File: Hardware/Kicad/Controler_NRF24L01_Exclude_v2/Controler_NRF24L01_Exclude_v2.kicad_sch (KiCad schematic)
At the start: 38 parts, among them J1 Conn_01x02, J2 Conn_02x07_Odd_Even, J3 Conn_01x03, J4 Conn_01x03, SW1 SW_Push, SW10 SW_Push, SW11 SW_DIP_x01, SW13 SW_DIP_x01, SW2 SW_Push, SW3 SW_Push, SW4 SW_Push, SW5 SW_Push, SW6 SW_Push, SW7 SW_Push, SW7 SW_SPST, SW8 SW_Push, SW9 SW_Push, U1 STM32L412KBTx, U2 MIC5219-3.3YMM, U2 nRF24_Full

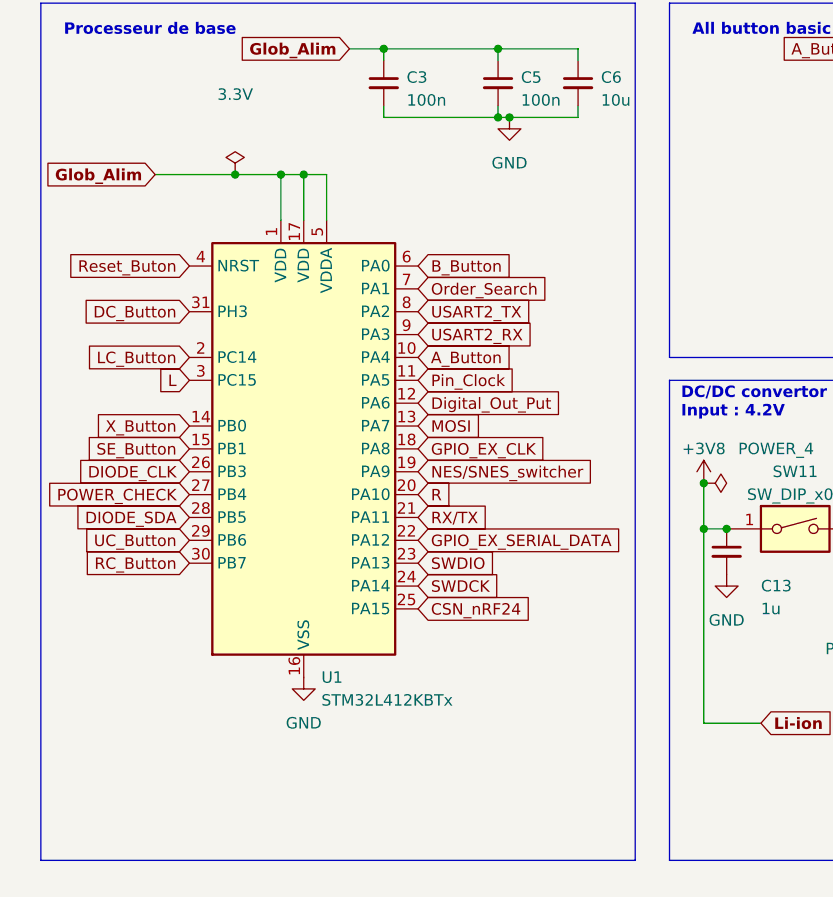
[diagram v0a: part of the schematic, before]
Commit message: V.2 controler
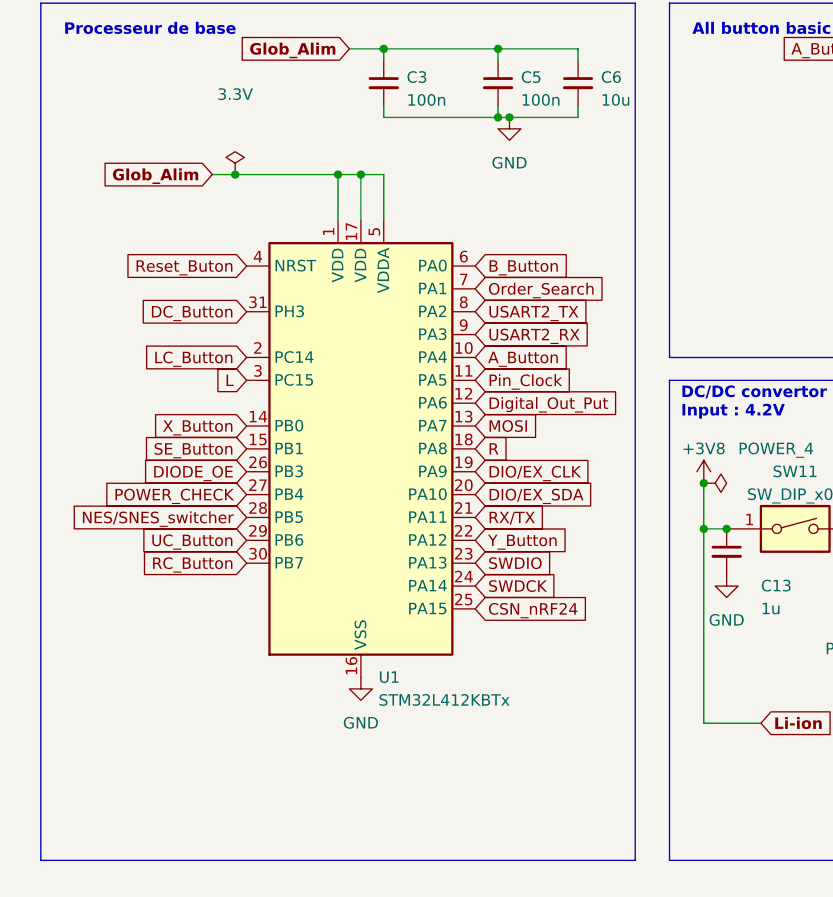
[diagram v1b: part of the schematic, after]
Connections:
- net DIODE_SDA is gone; now on net NES/SNES_switcher: U1.28 (PB5)
- net GPIO_EX_CLK is gone; now on net R: U1.18 (PA8)
- net GPIO_EX_SERIAL_DATA is gone; now on net Y_Button: U1.22 (PA12)
- net NES/SNES_switcher: no longer U1.19 (PA9)
- net R: no longer U1.20 (PA10)
- net DIODE_CLK renamed DIODE_OE
- new net DIO/EX_CLK: U1.19 (PA9)
- new net DIO/EX_SDA: U1.20 (PA10)
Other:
- moved on the sheet: U1

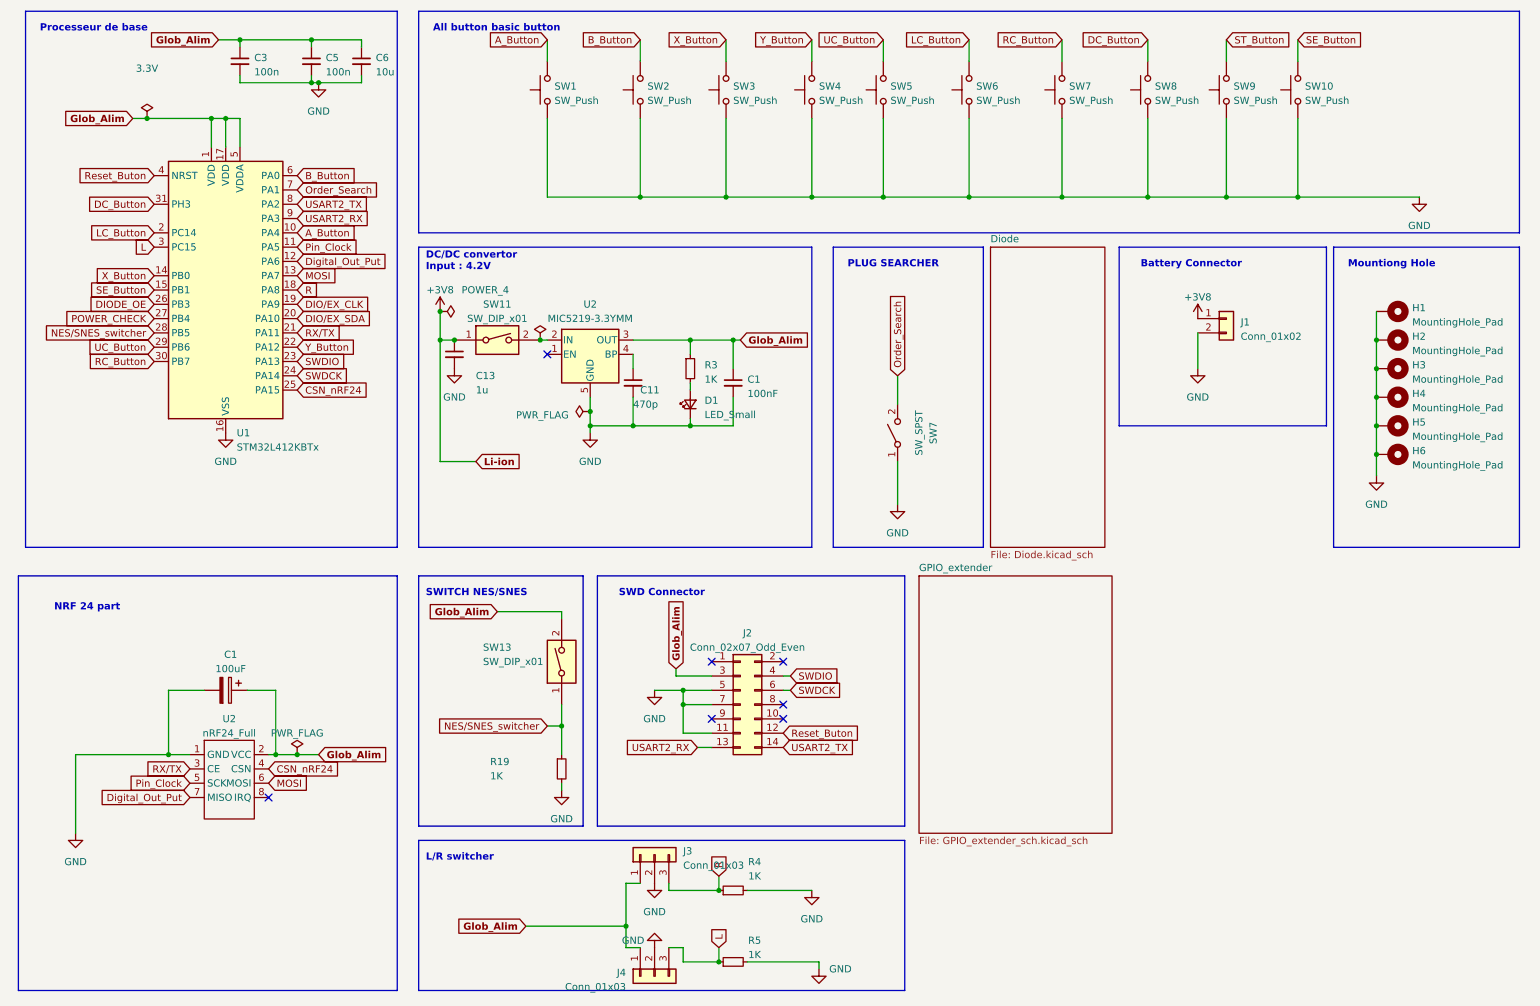
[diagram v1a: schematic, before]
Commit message: V.2 controler
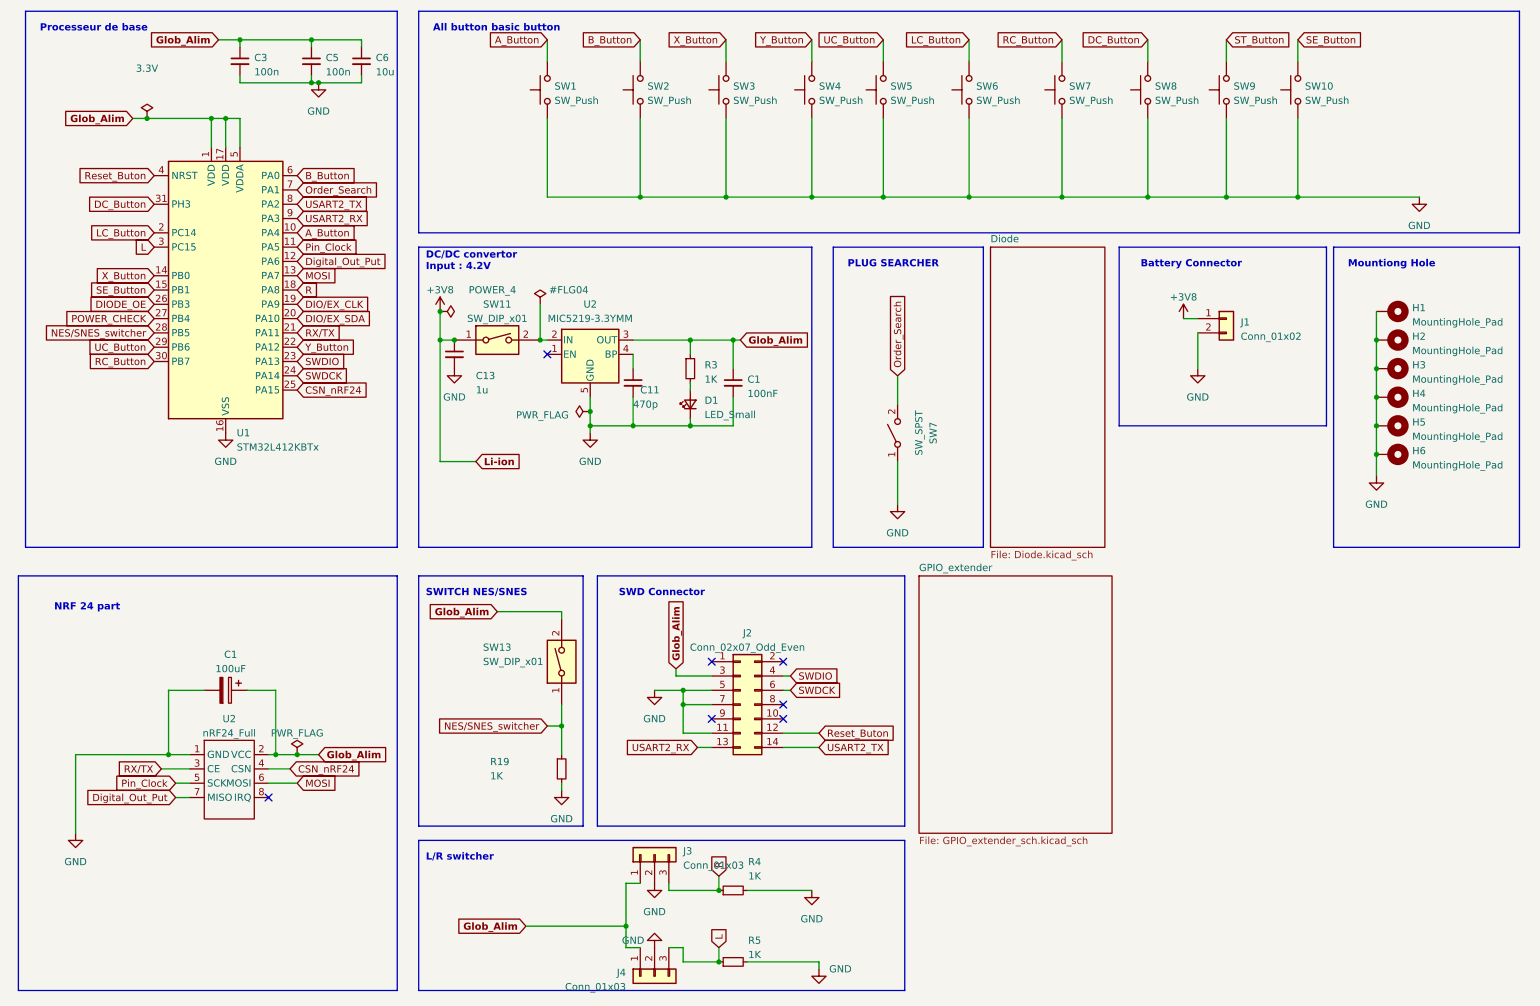
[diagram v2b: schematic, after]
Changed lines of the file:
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@@
+    (stroke (width 0) (type default))
+  )
+  (wire (pts (xy 39.37 149.86) (xy 44.45 149.86))
     (stroke (width 0) (type default))
   )
@@
     (stroke (width 0) (type default))
   )
+  (wire (pts (xy 63.5 152.4) (xy 58.42 152.4))
+    (stroke (width 0) (type default))
+  )
   (wire (pts (xy 143.51 171.45) (xy 154.94 171.45))
     (stroke (width 0) (type default))
@@
     (stroke (width 0) (type default))
   )
+  (wire (pts (xy 62.23 149.86) (xy 58.42 149.86))
+    (stroke (width 0) (type default))
+  )
   (wire (pts (xy 133.35 88.9) (xy 140.97 88.9))
     (stroke (width 0) (type default))
@@
     (stroke (width 0) (type default))
   )
+  (wire (pts (xy 41.91 154.94) (xy 44.45 154.94))
+    (stroke (width 0) (type default))
+  )
   (polyline (pts (xy 158.75 57.15) (xy 158.75 110.49))
     (stroke (width 0) (type default))
@@
     (stroke (width 0) (type default))
   )
+  (wire (pts (xy 41.91 152.4) (xy 44.45 152.4))
+    (stroke (width 0) (type default))
+  )
+  (wire (pts (xy 220.98 69.85) (xy 223.52 69.85))
+    (stroke (width 0) (type default))
+  )
   (wire (pts (xy 140.97 73.66) (xy 142.24 73.66))
     (stroke (width 0) (type default))
@@
     (stroke (width 0) (type default))
   )
+  (wire (pts (xy 156.21 146.05) (xy 149.86 146.05))
+    (stroke (width 0) (type default))
+  )
   (wire (pts (xy 228.6 20.32) (xy 228.6 24.13))
     (stroke (width 0) (type default))
@@
     (stroke (width 0) (type default))
   )
+  (wire (pts (xy 156.21 143.51) (xy 149.86 143.51))
+    (stroke (width 0) (type default))
+  )
   (wire (pts (xy 223.52 72.39) (xy 223.52 78.74))
     (stroke (width 0) (type default))
@@
   )
   (wire (pts (xy 104.14 177.8) (xy 121.92 177.8))
+    (stroke (width 0) (type default))
+  )
+  (wire (pts (xy 106.68 67.31) (xy 106.68 73.66))
     (stroke (width 0) (type default))
   )
@@
     )
   )
-  (global_label "Reset_Buton " (shape input) (at 149.86 143.51 0) (fields_autoplaced)
-    (effects (font (size 1.27 1.27)) (justify left))
-    (property "Intersheetrefs" "${INTERSHEET_REFS}" (at 165.1391 143.51 0)
+  (global_label "Reset_Buton " (shape input) (at 156.21 143.51 0) (fields_autoplaced)
+    (effects (font (size 1.27 1.27)) (justify left))
+    (property "Intersheetrefs" "${INTERSHEET_REFS}" (at 171.4891 143.51 0)
       (effects (font (size 1.27 1.27)) (justify left) hide)
     )
@@
     )
   )
-  (global_label "RX{slash}TX" (shape input) (at 44.45 149.86 180) (fields_autoplaced)
-    (effects (font (size 1.27 1.27)) (justify right))
-    (property "Intersheetrefs" "${INTERSHEET_REFS}" (at 35.5571 149.86 0)
+  (global_label "RX{slash}TX" (shape input) (at 39.37 149.86 180) (fields_autoplaced)
+    (effects (font (size 1.27 1.27)) (justify right))
+    (property "Intersheetrefs" "${INTERSHEET_REFS}" (at 30.4771 149.86 0)
       (effects (font (size 1.27 1.27)) (justify right) hide)
     )
@@
     )
   )
-  (global_label "USART2_TX" (shape input) (at 149.86 146.05 0) (fields_autoplaced)
-    (effects (font (size 1.27 1.27)) (justify left))
-    (property "Intersheetrefs" "${INTERSHEET_REFS}" (at 162.9862 146.05 0)
-      (effects (font (size 1.27 1.27)) (justify left) hide)
-    )
-  )
-  (global_label "Pin_Clock" (shape input) (at 44.45 152.4 180) (fields_autoplaced)
-    (effects (font (size 1.27 1.27)) (justify right))
-    (property "Intersheetrefs" "${INTERSHEET_REFS}" (at 32.3519 152.4 0)
+  (global_label "USART2_TX" (shape input) (at 156.21 146.05 0) (fields_autoplaced)
+    (effects (font (size 1.27 1.27)) (justify left))
+    (property "Intersheetrefs" "${INTERSHEET_REFS}" (at 169.3362 146.05 0)
+      (effects (font (size 1.27 1.27)) (justify left) hide)
+    )
+  )
+  (global_label "Pin_Clock" (shape input) (at 41.91 152.4 180) (fields_autoplaced)
+    (effects (font (size 1.27 1.27)) (justify right))
+    (property "Intersheetrefs" "${INTERSHEET_REFS}" (at 29.8119 152.4 0)
       (effects (font (size 1.27 1.27)) (justify right) hide)
     )
@@
     )
   )
-  (global_label "Digital_Out_Put" (shape input) (at 44.45 154.94 180) (fields_autoplaced)
-    (effects (font (size 1.27 1.27)) (justify right))
-    (property "Intersheetrefs" "${INTERSHEET_REFS}" (at 27.0906 154.94 0)
+  (global_label "Digital_Out_Put" (shape input) (at 41.91 154.94 180) (fields_autoplaced)
+    (effects (font (size 1.27 1.27)) (justify right))
+    (property "Intersheetrefs" "${INTERSHEET_REFS}" (at 24.5506 154.94 0)
       (effects (font (size 1.27 1.27)) (justify right) hide)
     )
@@
     )
   )
-  (global_label "MOSI" (shape input) (at 58.42 152.4 0) (fields_autoplaced)
-    (effects (font (size 1.27 1.27)) (justify left))
-    (property "Intersheetrefs" "${INTERSHEET_REFS}" (at 65.922 152.4 0)
+  (global_label "MOSI" (shape input) (at 63.5 152.4 0) (fields_autoplaced)
+    (effects (font (size 1.27 1.27)) (justify left))
+    (property "Intersheetrefs" "${INTERSHEET_REFS}" (at 71.002 152.4 0)
       (effects (font (size 1.27 1.27)) (justify left) hide)
     )
@@
     )
   )
-  (global_label "CSN_nRF24" (shape input) (at 58.42 149.86 0) (fields_autoplaced)
-    (effects (font (size 1.27 1.27)) (justify left))
-    (property "Intersheetrefs" "${INTERSHEET_REFS}" (at 72.03 149.86 0)
+  (global_label "CSN_nRF24" (shape input) (at 62.23 149.86 0) (fields_autoplaced)
+    (effects (font (size 1.27 1.27)) (justify left))
+    (property "Intersheetrefs" "${INTERSHEET_REFS}" (at 75.84 149.86 0)
       (effects (font (size 1.27 1.27)) (justify left) hide)
     )
@@
     )
   )
-  (symbol (lib_id "power:PWR_FLAG") (at 106.68 73.66 0) (unit 1)
+  (symbol (lib_id "power:PWR_FLAG") (at 106.68 67.31 0) (unit 1)
     (in_bom yes) (on_board yes) (dnp no)
-    (property "Reference" "#FLG04" (at 106.68 71.755 0)
-      (effects (font (size 1.27 1.27)) hide)
-    )
-    (property "Value" "3.8V" (at 106.68 64.77 0)
-      (effects (font (size 1.27 1.27)) hide)
-    )
-    (property "Footprint" "" (at 106.68 73.66 0)
-      (effects (font (size 1.27 1.27)) hide)
-    )
-    (property "Datasheet" "~" (at 106.68 73.66 0)
+    (property "Reference" "#FLG04" (at 111.76 64.77 0)
+      (effects (font (size 1.27 1.27)))
+    )
+    (property "Value" "3.8V" (at 106.68 58.42 0)
+      (effects (font (size 1.27 1.27)) hide)
+    )
+    (property "Footprint" "" (at 106.68 67.31 0)
+      (effects (font (size 1.27 1.27)) hide)
+    )
+    (property "Datasheet" "~" (at 106.68 67.31 0)
       (effects (font (size 1.27 1.27)) hide)
     )
@@
       (project "Controler_NRF24L01_Exclude_v2"
         (path "/76ef48f1-60b7-4c4b-a0ce-73b6af33b115"
-          (reference "#FLG05") (unit 1)
+          (reference "FLG05") (unit 1)
         )
       )
@@
     )
   )
-  (symbol (lib_id "power:+3V8") (at 223.52 69.85 0) (unit 1)
-    (in_bom yes) (on_board yes) (dnp no) (fields_autoplaced)
-    (property "Reference" "#PWR05" (at 223.52 73.66 0)
-      (effects (font (size 1.27 1.27)) hide)
-    )
-    (property "Value" "+3V8" (at 223.52 66.04 0)
-      (effects (font (size 1.27 1.27)))
-    )
-    (property "Footprint" "" (at 223.52 69.85 0)
-      (effects (font (size 1.27 1.27)) hide)
-    )
-    (property "Datasheet" "" (at 223.52 69.85 0)
+  (symbol (lib_id "power:+3V8") (at 220.98 69.85 0) (unit 1)
+    (in_bom yes) (on_board yes) (dnp no) (fields_autoplaced)
+    (property "Reference" "#PWR05" (at 220.98 73.66 0)
+      (effects (font (size 1.27 1.27)) hide)
+    )
+    (property "Value" "+3V8" (at 220.98 66.04 0)
+      (effects (font (size 1.27 1.27)))
+    )
+    (property "Footprint" "" (at 220.98 69.85 0)
+      (effects (font (size 1.27 1.27)) hide)
+    )
+    (property "Datasheet" "" (at 220.98 69.85 0)
       (effects (font (size 1.27 1.27)) hide)
     )
@@
       (effects (font (size 1.27 1.27)) hide)
     )
-    (property "Value" "POWER_4" (at 92.71 64.77 90)
-      (effects (font (size 1.27 1.27)) (justify left))
-    )
+    (property "Value" "POWER_4" (at 93.98 64.77 90)
+      (effects (font (size 1.27 1.27)) (justify left))
+    )
